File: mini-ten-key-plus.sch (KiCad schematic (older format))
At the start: 65 parts, among them SW0 SW_Push, U0 ProMicro

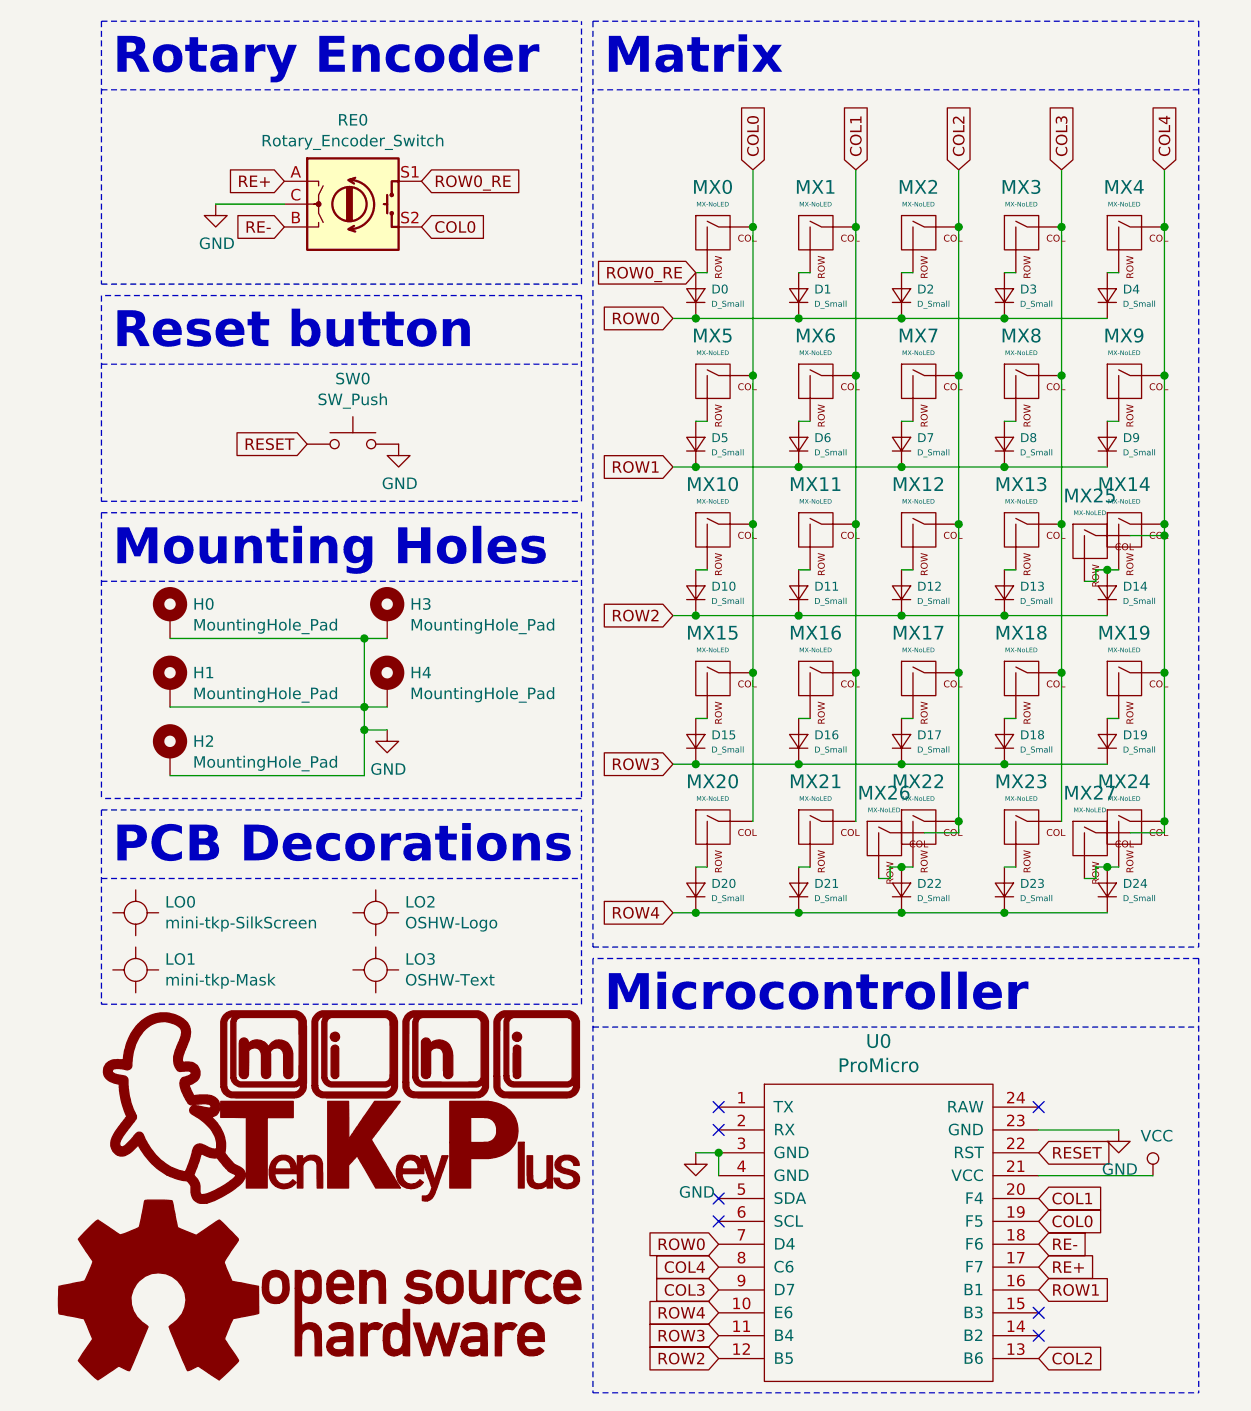
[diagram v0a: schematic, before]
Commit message: Added layout image and general edits
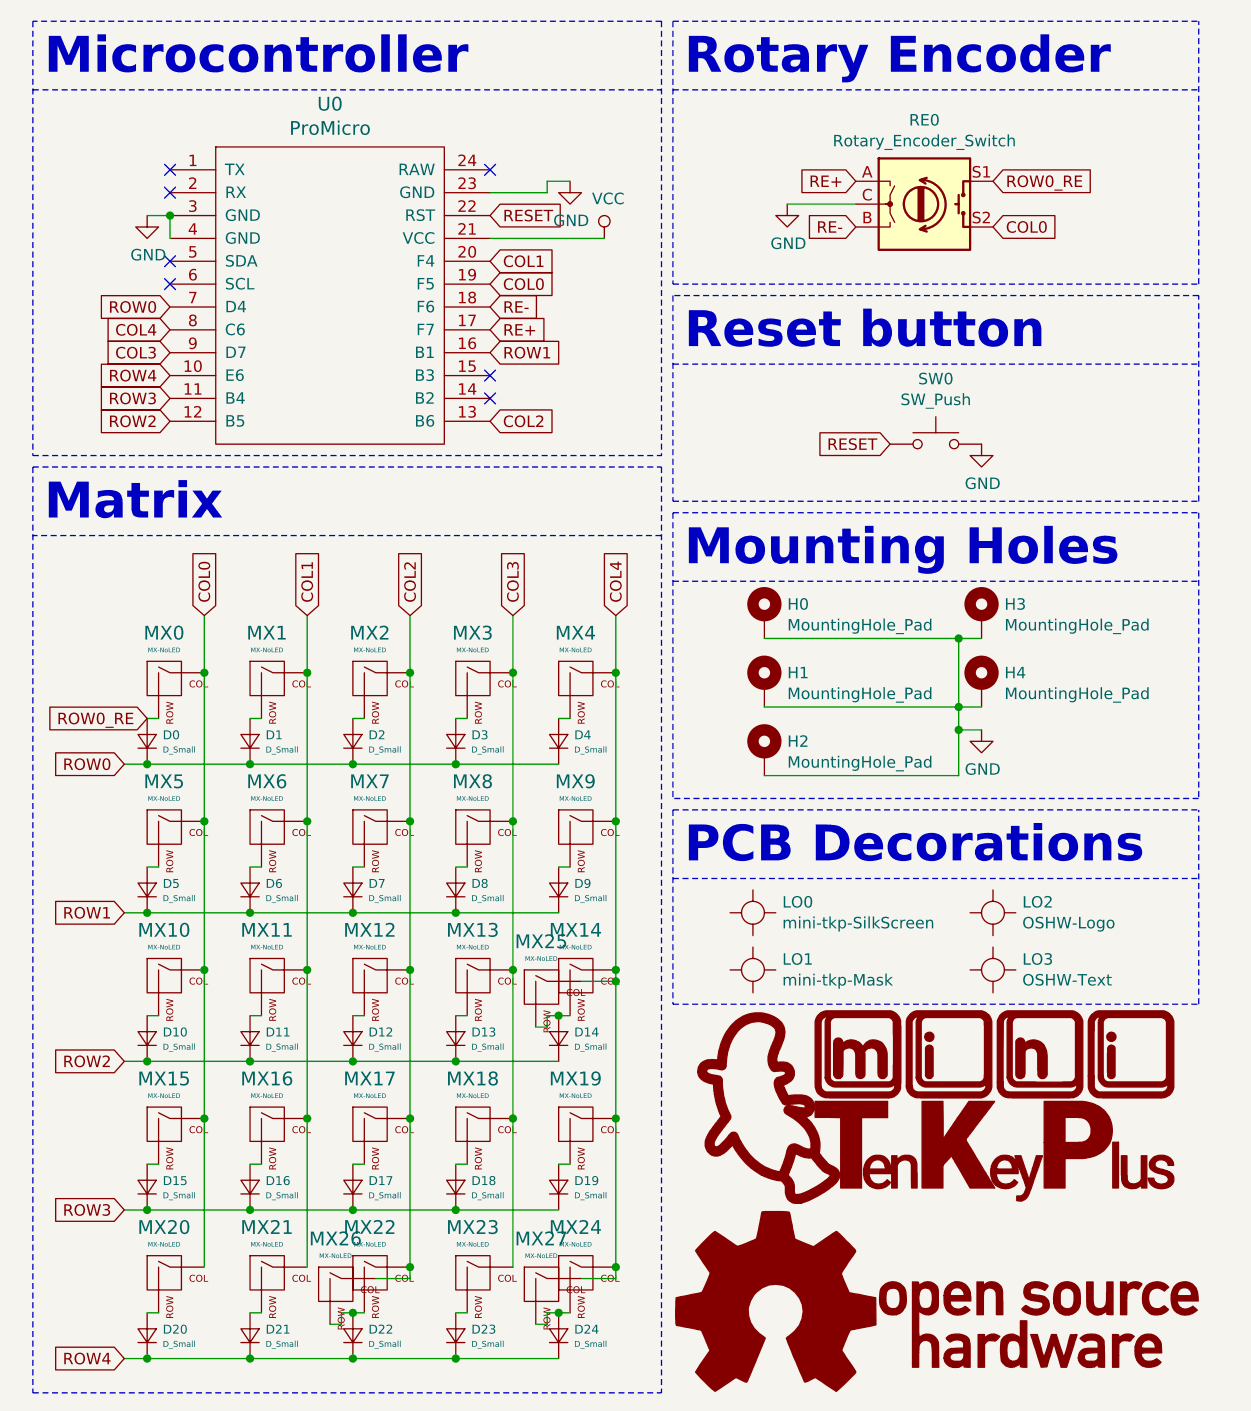
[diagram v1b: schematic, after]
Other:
- moved on the sheet: D0, D1, D10, D11, D12, D13, D14, D15, D16, D17, D18, D19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

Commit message: Added LICENSE
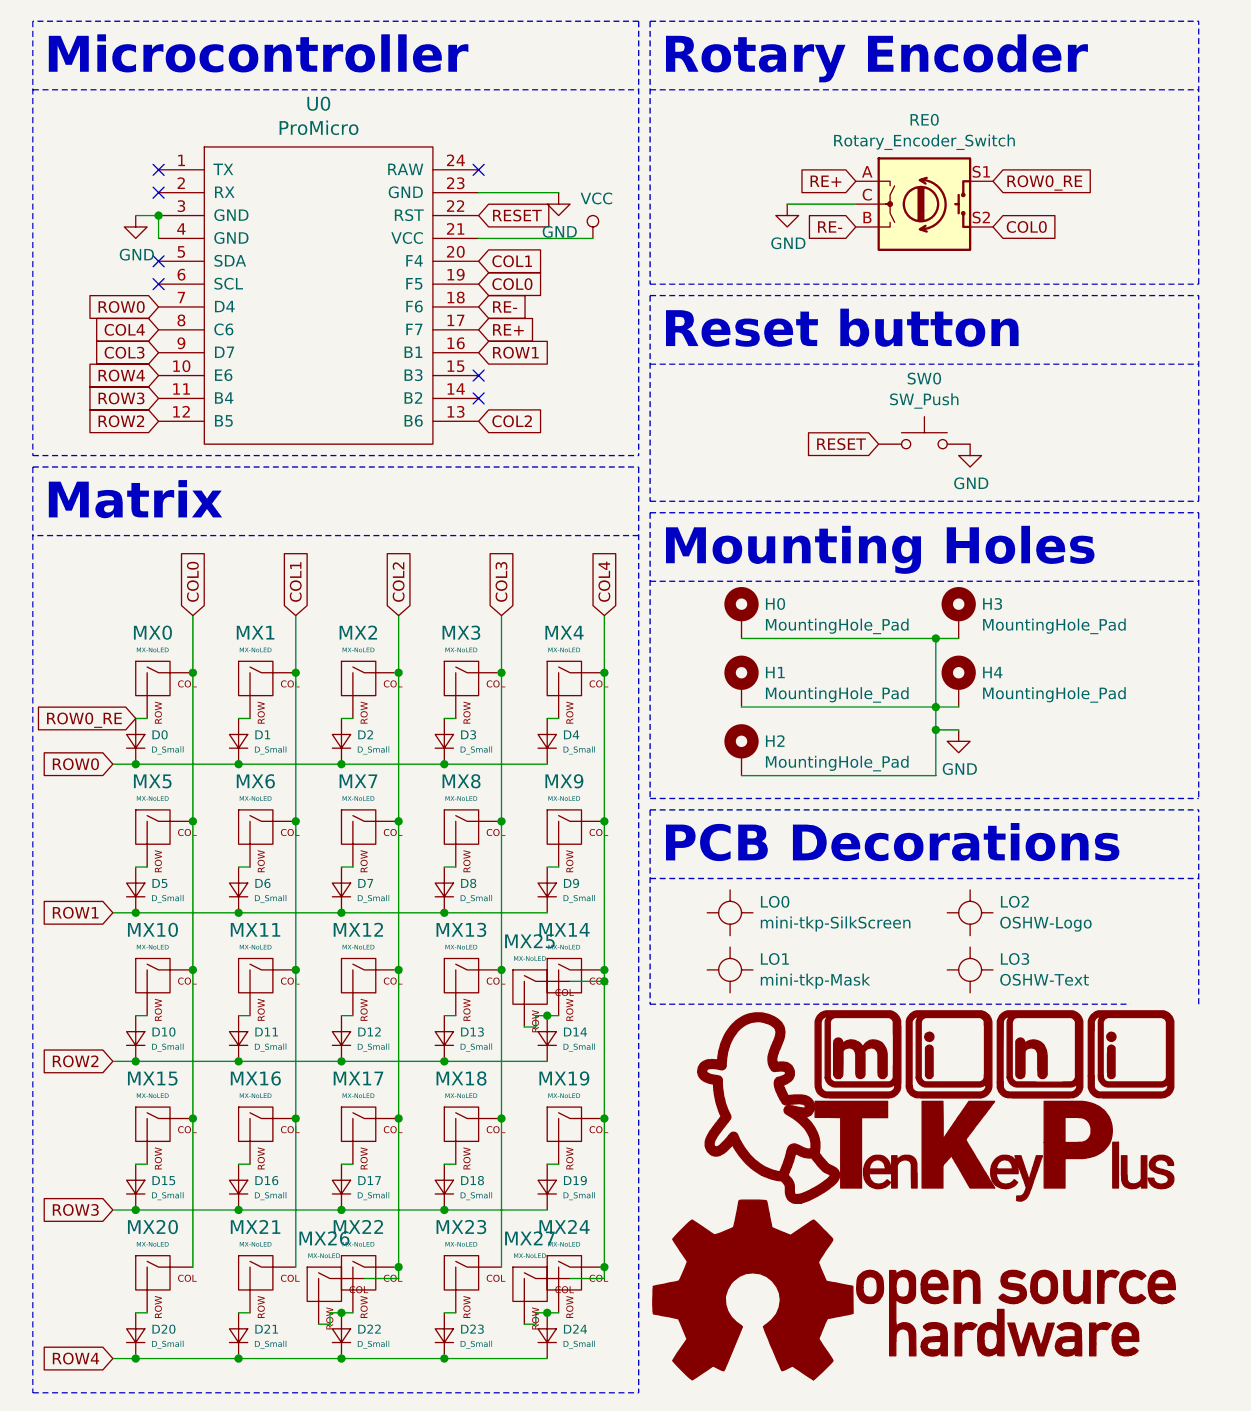
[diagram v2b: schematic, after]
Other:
- moved on the sheet: D0, D1, D10, D11, D12, D13, D14, D15, D16, D17, D18, D19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
